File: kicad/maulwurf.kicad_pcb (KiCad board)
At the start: 2 copper layers, 63.5 x 70 mm, 18 parts

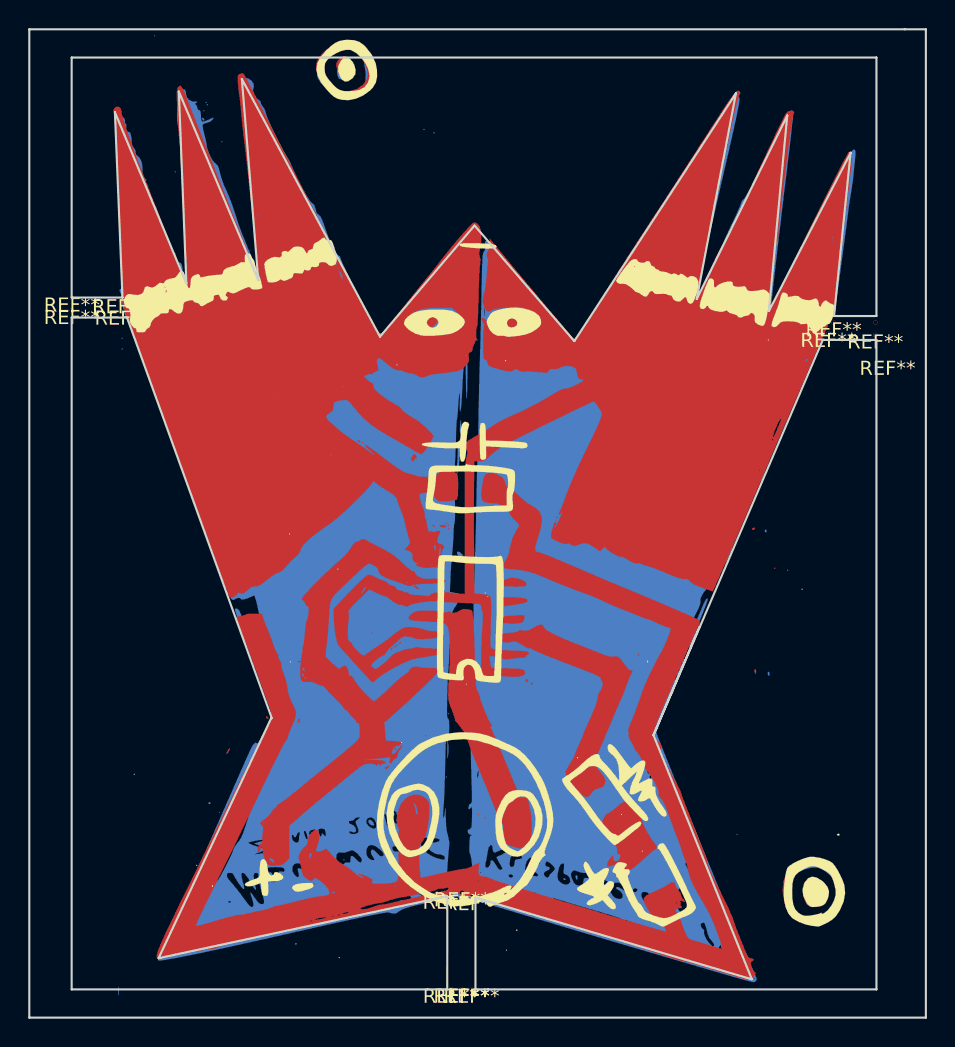
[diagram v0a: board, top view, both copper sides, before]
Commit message: Improve rat-bites
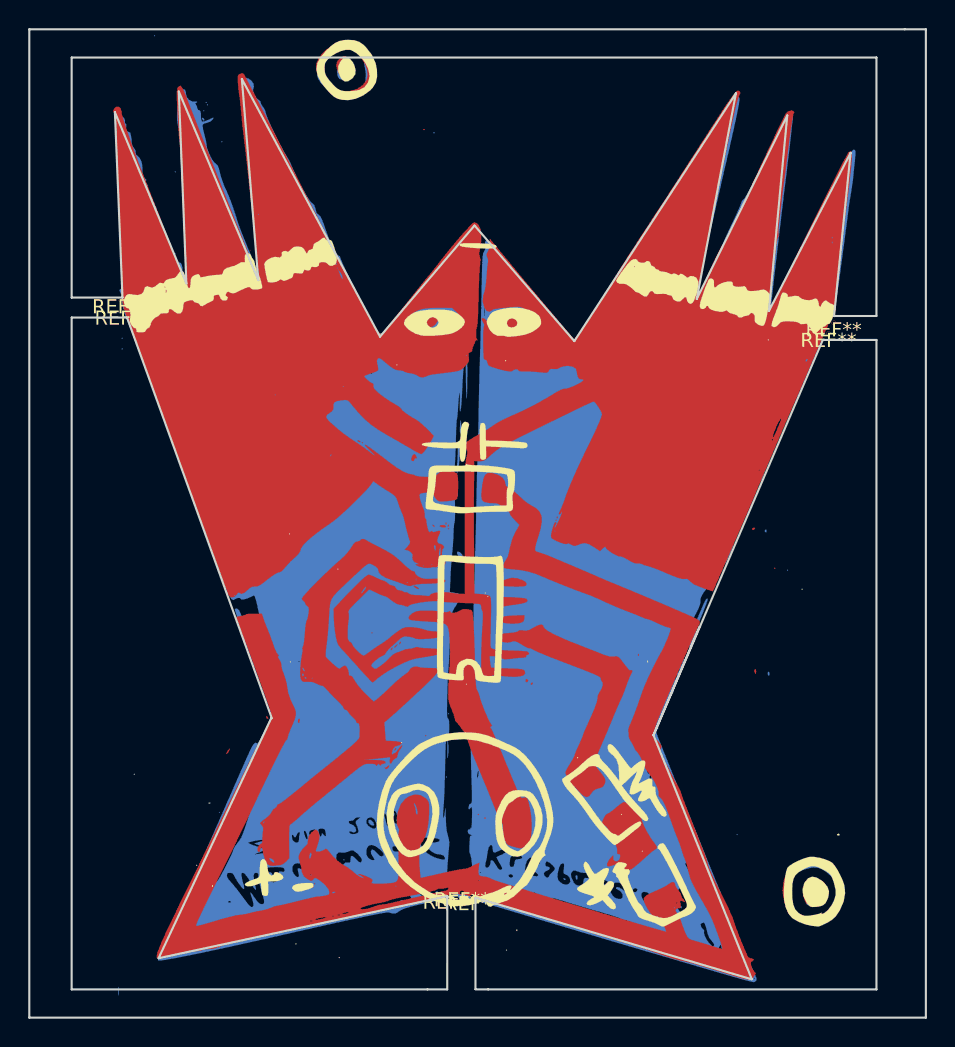
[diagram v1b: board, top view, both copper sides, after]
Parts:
- removed the REF** at (139.3, 128.0)
- removed the REF** at (167.9, 81.6)
- removed the REF** at (167.9, 80.8)
- removed the REF** at (111.0, 79.9)
- removed the REF** at (111.0, 79.0)
- removed the REF** at (137.9, 128.0)
- removed the REF** at (138.6, 128.0)
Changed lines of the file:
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@@
     (tracks 1)
     (zones 0)
-    (modules 18)
+    (modules 11)
     (nets 1)
   )
@@
   )
   (module footprints:hole (layer F.Cu)
-    (at 111.016 79.912)
-    (fp_text reference REF** (at 0 0.5) (layer F.SilkS)
-      (effects (font (size 1 1) (thickness 0.15)))
-    )
-    (fp_text value hole (at 0 -0.5) (layer F.Fab)
-      (effects (font (size 1 1) (thickness 0.15)))
-    )
-    (pad 1 thru_hole circle (at 0 0) (size 0.3 0.3) (drill 0.3) (layers *.Cu *.Mask))
-  )
-  (module footprints:hole (layer F.Cu)
-    (at 111.019 79.033)
-    (fp_text reference REF** (at 0 0.5) (layer F.SilkS)
-      (effects (font (size 1 1) (thickness 0.15)))
-    )
-    (fp_text value hole (at 0 -0.5) (layer F.Fab)
-      (effects (font (size 1 1) (thickness 0.15)))
-    )
-    (pad 1 thru_hole circle (at 0 0) (size 0.3 0.3) (drill 0.3) (layers *.Cu *.Mask))
-  )
-  (module footprints:hole (layer F.Cu)
     (at 114.434 79.151)
     (fp_text reference REF** (at 0 0.5) (layer F.SilkS)
@@
       (effects (font (size 1 1) (thickness 0.15)))
     )
-    (fp_text value hole (at 0 -0.5) (layer F.Fab)
-      (effects (font (size 1 1) (thickness 0.15)))
-    )
-    (pad 1 thru_hole circle (at 0 0) (size 0.3 0.3) (drill 0.3) (layers *.Cu *.Mask))
-  )
-  (module footprints:hole (layer F.Cu)
-    (at 137.861 127.986)
-    (fp_text reference REF** (at 0 0.5) (layer F.SilkS)
-      (effects (font (size 1 1) (thickness 0.15)))
-    )
-    (fp_text value hole (at 0 -0.5) (layer F.Fab)
-      (effects (font (size 1 1) (thickness 0.15)))
-    )
-    (pad 1 thru_hole circle (at 0 0) (size 0.3 0.3) (drill 0.3) (layers *.Cu *.Mask))
-  )
-  (module footprints:hole (layer F.Cu)
-    (at 138.612 127.977)
-    (fp_text reference REF** (at 0 0.5) (layer F.SilkS)
-      (effects (font (size 1 1) (thickness 0.15)))
-    )
-    (fp_text value hole (at 0 -0.5) (layer F.Fab)
-      (effects (font (size 1 1) (thickness 0.15)))
-    )
-    (pad 1 thru_hole circle (at 0 0) (size 0.3 0.3) (drill 0.3) (layers *.Cu *.Mask))
-  )
-  (module footprints:hole (layer F.Cu)
-    (at 139.322 127.986)
-    (fp_text reference REF** (at 0 0.5) (layer F.SilkS)
-      (effects (font (size 1 1) (thickness 0.15)))
-    )
-    (fp_text value hole (at 0 -0.5) (layer F.Fab)
-      (effects (font (size 1 1) (thickness 0.15)))
-    )
-    (pad 1 thru_hole circle (at 0 0) (size 0.3 0.3) (drill 0.3) (layers *.Cu *.Mask))
-  )
-  (module footprints:hole (layer F.Cu)
-    (at 167.916 81.645)
-    (fp_text reference REF** (at 0 0.5) (layer F.SilkS)
-      (effects (font (size 1 1) (thickness 0.15)))
-    )
-    (fp_text value hole (at 0 -0.5) (layer F.Fab)
-      (effects (font (size 1 1) (thickness 0.15)))
-    )
-    (pad 1 thru_hole circle (at 0 0) (size 0.3 0.3) (drill 0.3) (layers *.Cu *.Mask))
-  )
-  (module footprints:hole (layer F.Cu)
-    (at 167.93 80.758)
-    (fp_text reference REF** (at 0.855 3.254) (layer F.SilkS)
-      (effects (font (size 1 1) (thickness 0.15)))
-    )

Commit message: Improve the frame
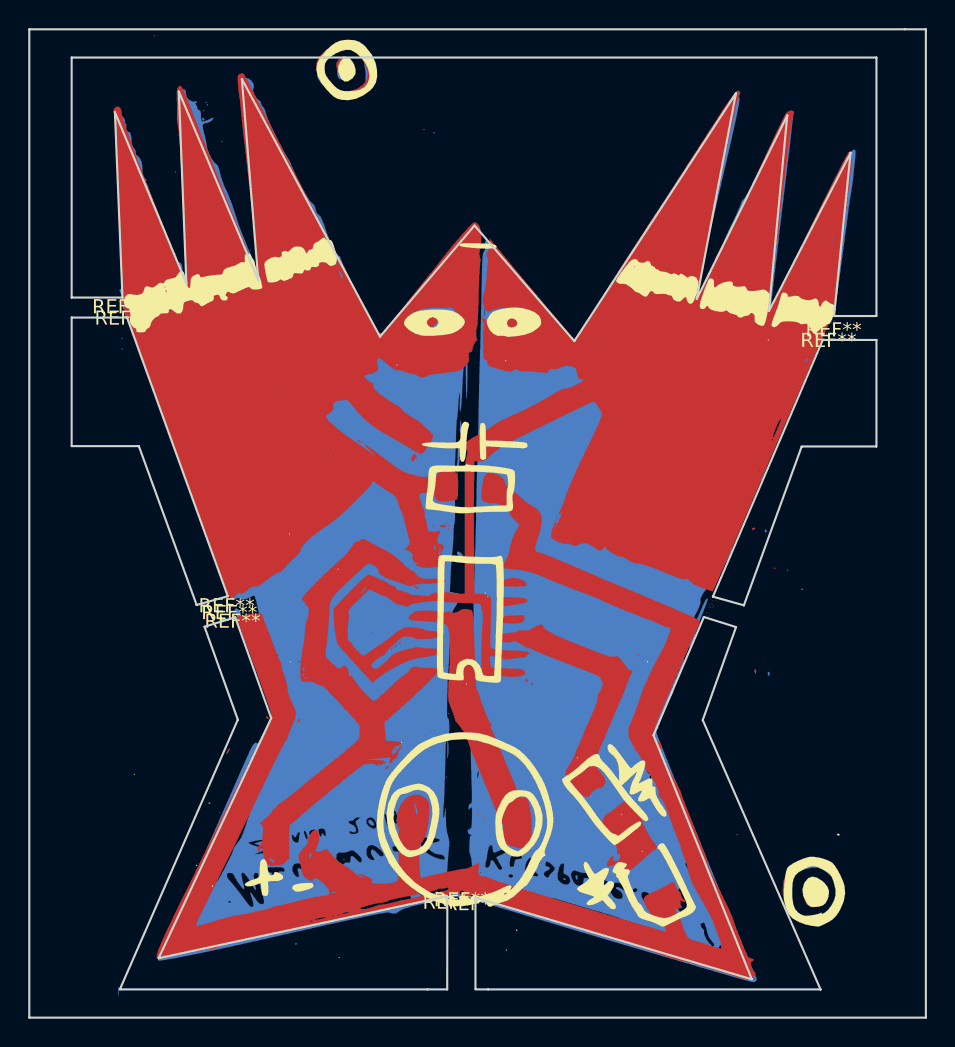
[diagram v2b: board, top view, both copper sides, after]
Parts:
- added REF**: hole, footprints:hole, B.Cu at (156.5, 100.4)
- added REF**: hole, footprints:hole, B.Cu at (156.1, 101.4)
- added REF**: hole, footprints:hole, B.Cu at (156.3, 100.8)
- added REF**: hole, footprints:hole, F.Cu at (122.0, 100.3)
- added REF**: hole, footprints:hole, F.Cu at (122.4, 101.4)
- added REF**: hole, footprints:hole, F.Cu at (122.2, 100.8)
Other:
- outline, holes or cut-outs redrawn
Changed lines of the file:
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@@
     (links 0)
     (no_connects 0)
-    (area 107.924999 55.664333 171.575001 130.075001)
+    (area 107.924999 59.924999 171.575001 130.075001)
     (thickness 1.6)
-    (drawings 44)
+    (drawings 57)
     (tracks 1)
     (zones 0)
-    (modules 11)
+    (modules 17)
     (nets 1)
   )
@@
     (35 F.Paste user hide)
     (36 B.SilkS user hide)
-    (37 F.SilkS user)
+    (37 F.SilkS user hide)
     (38 B.Mask user hide)
-    (39 F.Mask user hide)
+    (39 F.Mask user)
     (40 Dwgs.User user hide)
     (41 Cmts.User user hide)
@@
     (uvia_drill 0.1)
   )
+  (module footprints:hole (layer B.Cu)
+    (at 156.489477 100.350167 180)
+    (fp_text reference REF** (at 0 -0.5 180) (layer B.SilkS)
+      (effects (font (size 1 1) (thickness 0.15)) (justify mirror))
+    )
+    (fp_text value hole (at 0 0.5 180) (layer B.Fab)
+      (effects (font (size 1 1) (thickness 0.15)) (justify mirror))
+    )
+    (pad 1 thru_hole circle (at 0 0 180) (size 0.3 0.3) (drill 0.3) (layers *.Cu *.Mask))
+  )
+  (module footprints:hole (layer B.Cu)
+    (at 156.071477 101.446167 180)
+    (fp_text reference REF** (at 0 -0.5 180) (layer B.SilkS)
+      (effects (font (size 1 1) (thickness 0.15)) (justify mirror))
+    )
+    (fp_text value hole (at 0 0.5 180) (layer B.Fab)
+      (effects (font (size 1 1) (thickness 0.15)) (justify mirror))
+    )
+    (pad 1 thru_hole circle (at 0 0 180) (size 0.3 0.3) (drill 0.3) (layers *.Cu *.Mask))
+  )
+  (module footprints:hole (layer B.Cu)
+    (at 156.298477 100.837167 180)
+    (fp_text reference REF** (at 0 -0.5 180) (layer B.SilkS)
+      (effects (font (size 1 1) (thickness 0.15)) (justify mirror))
+    )
+    (fp_text value hole (at 0 0.5 180) (layer B.Fab)
+      (effects (font (size 1 1) (thickness 0.15)) (justify mirror))
+    )
+    (pad 1 thru_hole circle (at 0 0 180) (size 0.3 0.3) (drill 0.3) (layers *.Cu *.Mask))
+  )
+  (module footprints:hole (layer F.Cu)
+    (at 121.976 100.325)
+    (fp_text reference REF** (at 0 0.5) (layer F.SilkS)
+      (effects (font (size 1 1) (thickness 0.15)))
+    )
+    (fp_text value hole (at 0 -0.5) (layer F.Fab)
+      (effects (font (size 1 1) (thickness 0.15)))
+    )
+    (pad 1 thru_hole circle (at 0 0) (size 0.3 0.3) (drill 0.3) (layers *.Cu *.Mask))
+  )
+  (module footprints:hole (layer F.Cu)
+    (at 122.394 101.421)
+    (fp_text reference REF** (at 0 0.5) (layer F.SilkS)
+      (effects (font (size 1 1) (thickness 0.15)))
+    )
+    (fp_text value hole (at 0 -0.5) (layer F.Fab)
+      (effects (font (size 1 1) (thickness 0.15)))
+    )
+    (pad 1 thru_hole circle (at 0 0) (size 0.3 0.3) (drill 0.3) (layers *.Cu *.Mask))
+  )
+  (module footprints:hole (layer F.Cu)
+    (at 122.167 100.812)
+    (fp_text reference REF** (at 0 0.5) (layer F.SilkS)
+      (effects (font (size 1 1) (thickness 0.15)))
+    )
+    (fp_text value hole (at 0 -0.5) (layer F.Fab)
+      (effects (font (size 1 1) (thickness 0.15)))
+    )
+    (pad 1 thru_hole circle (at 0 0) (size 0.3 0.3) (drill 0.3) (layers *.Cu *.Mask))
+  )
   (module footprints:mask (layer F.Cu)
     (at 163.658 121.284)
@@
       (xy -32.213849 -59.695039) (xy -31.985009 -59.594131)) (layer F.SilkS) (width 0.01))
   )
-  (gr_line (start 152.216 109.984) (end 155.456 102.324) (layer Edge.Cuts) (width 0.15))
+  (gr_line (start 162.700477 89.563167) (end 158.606477 100.812167) (layer Edge.Cuts) (width 0.15))
+  (gr_line (start 167.978227 89.547167) (end 162.700412 89.547167) (angle 90) (layer Edge.Cuts) (width 0.15))
+  (gr_line (start 158.625477 100.800167) (end 156.407477 100.180167) (layer Edge.Cuts) (width 0.15))
+  (gr_line (start 155.691477 108.934167) (end 158.056477 102.339167) (layer Edge.Cuts) (width 0.15))
+  (gr_line (start 155.777 101.622) (end 158.055477 102.338167) (layer Edge.Cuts) (width 0.15))
+  (gr_line (start 155.698477 108.926167) (end 164.047477 128.017167) (layer Edge.Cuts) (width 0.15))
+  (gr_line (start 125.131 108.783) (end 122.586 101.65) (layer Edge.Cuts) (width 0.15))
+  (gr_line (start 122.774 108.909) (end 120.409 102.314) (layer Edge.Cuts) (width 0.15))
+  (gr_line (start 122.584 101.648) (end 120.41 102.313) (layer Edge.Cuts) (width 0.15))
+  (gr_line (start 119.84 100.775) (end 122.058 100.155) (layer Edge.Cuts) (width 0.15))
+  (gr_line (start 122.767 108.901) (end 114.418 127.992) (layer Edge.Cuts) (width 0.15))
+  (gr_line (start 115.765 89.538) (end 119.859 100.787) (layer Edge.Cuts) (width 0.15))
+  (gr_line (start 111.004979 89.522) (end 115.765065 89.522) (angle 90) (layer Edge.Cuts) (width 0.15))
+  (gr_line (start 152.216 109.984) (end 155.779 101.622) (layer Edge.Cuts) (width 0.15))
   (gr_line (start 171.5 60) (end 170 60) (layer Edge.Cuts) (width 0.15))
   (gr_line (start 171.5 130) (end 171.5 60) (layer Edge.Cuts) (width 0.15))
@@
   (gr_line (start 140.4 128) (end 140.5 128) (layer F.Mask) (width 0.2))
   (gr_line (start 139.6 128) (end 140.4 128) (layer F.Mask) (width 0.2))
-  (gr_line (start 111 128) (end 136.2 128) (layer Edge.Cuts) (width 0.15))
+  (gr_line (start 114.410909 128) (end 136.2 128) (layer Edge.Cuts) (width 0.15))
   (gr_line (start 139.6 121.499) (end 139.6 127.977) (layer Edge.Cuts) (width 0.15))
   (gr_line (start 137.6 128) (end 137.607 121.399) (layer Edge.Cuts) (width 0.15))
   (gr_line (start 168 62) (end 111 62) (layer Edge.Cuts) (width 0.15))
-  (gr_line (start 168 128) (end 168 82) (layer Edge.Cuts) (width 0.15))
-  (gr_line (start 140.5 128) (end 168 128) (layer Edge.Cuts) (width 0.15))
-  (gr_line (start 111 80.409988) (end 111 128) (layer Edge.Cuts) (width 0.15))
+  (gr_line (start 168 89.554279) (end 168 82) (layer Edge.Cuts) (width 0.15))
+  (gr_line (start 140.5 128) (end 164.04501 128) (layer Edge.Cuts) (width 0.15))
+  (gr_line (start 111 80.409988) (end 111 89.525) (layer Edge.Cuts) (width 0.15))
   (gr_line (start 117.158 125.793) (end 125.138 108.784) (layer Edge.Cuts) (width 0.15))
   (gr_line (start 137.6 121.4) (end 117.158 125.793) (layer Edge.Cuts) (width 0.15))
   (gr_line (start 159.174 127.286) (end 139.6 121.5) (layer Edge.Cuts) (width 0.15))
   (gr_line (start 152.205 109.981) (end 159.174 127.286) (layer Edge.Cuts) (width 0.15))
-  (gr_line (start 164.201 82) (end 152.202 110) (layer Edge.Cuts) (width 0.15))
+  (gr_line (start 164.201 82) (end 156.417 100.184) (layer Edge.Cuts) (width 0.15))
   (gr_line (start 166.169 68.752) (end 164.996 80.308) (layer Edge.Cuts) (width 0.15))
   (gr_line (start 160.381 79.955) (end 166.169 68.752) (layer Edge.Cuts) (width 0.15))
@@
   (gr_line (start 114.062 65.872) (end 119.124 77.993) (layer Edge.Cuts) (width 0.15))
   (gr_line (start 114.6 79) (end 114.062 65.872) (layer Edge.Cuts) (width 0.15))
-  (gr_line (start 125.177 108.797) (end 114.923 80.41) (layer Edge.Cuts) (width 0.15))
+  (gr_line (start 122.06 100.157) (end 114.923 80.41) (layer Edge.Cuts) (width 0.15))
   (segment (start 139.193 98.182) (end 139.193 100.299) (width 0.25) (layer F.Cu) (net 0))
   (zone (net 0) (net_name "") (layer B.Mask) (hatch edge 0.508)
